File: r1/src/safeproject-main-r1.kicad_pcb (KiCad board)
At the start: 2 copper layers, 29 x 46.5 mm, 18 parts, among them J1 2842142-4, J2 Conn_01x20

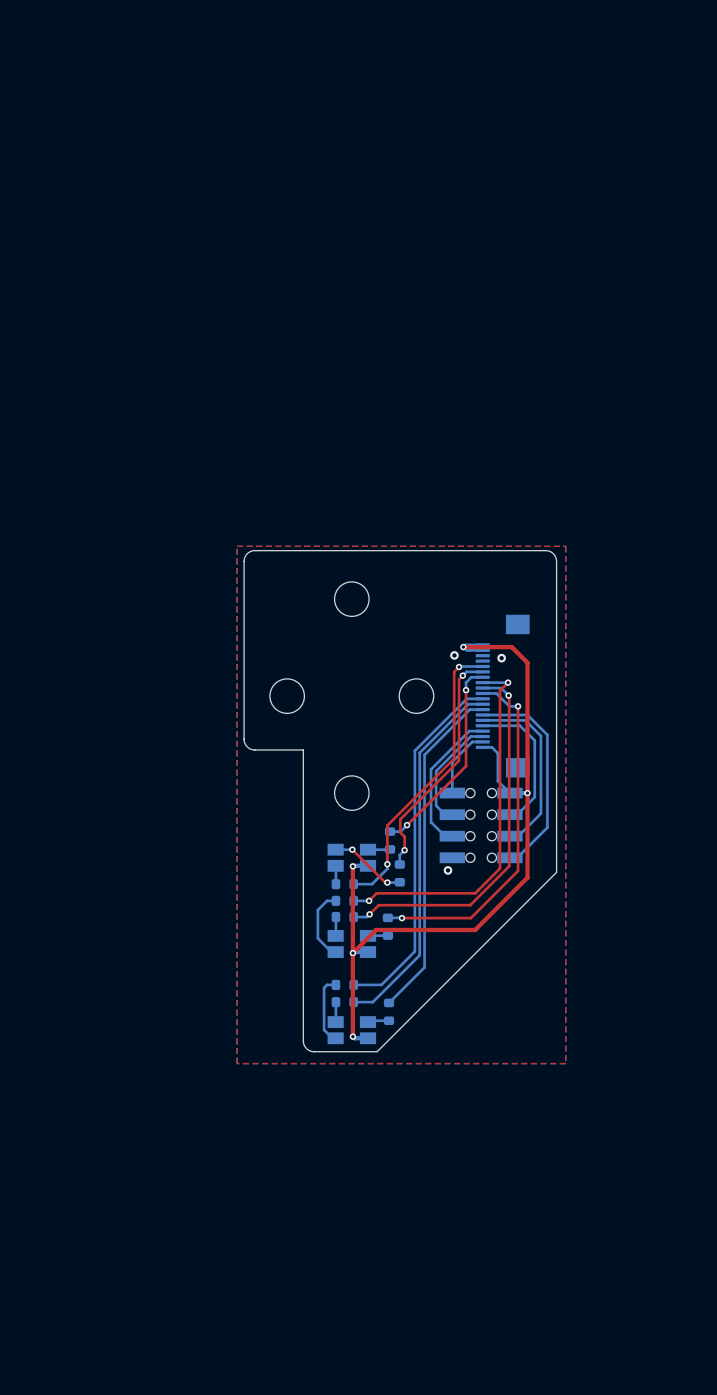
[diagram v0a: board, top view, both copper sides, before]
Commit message: Board routed, DRC pass
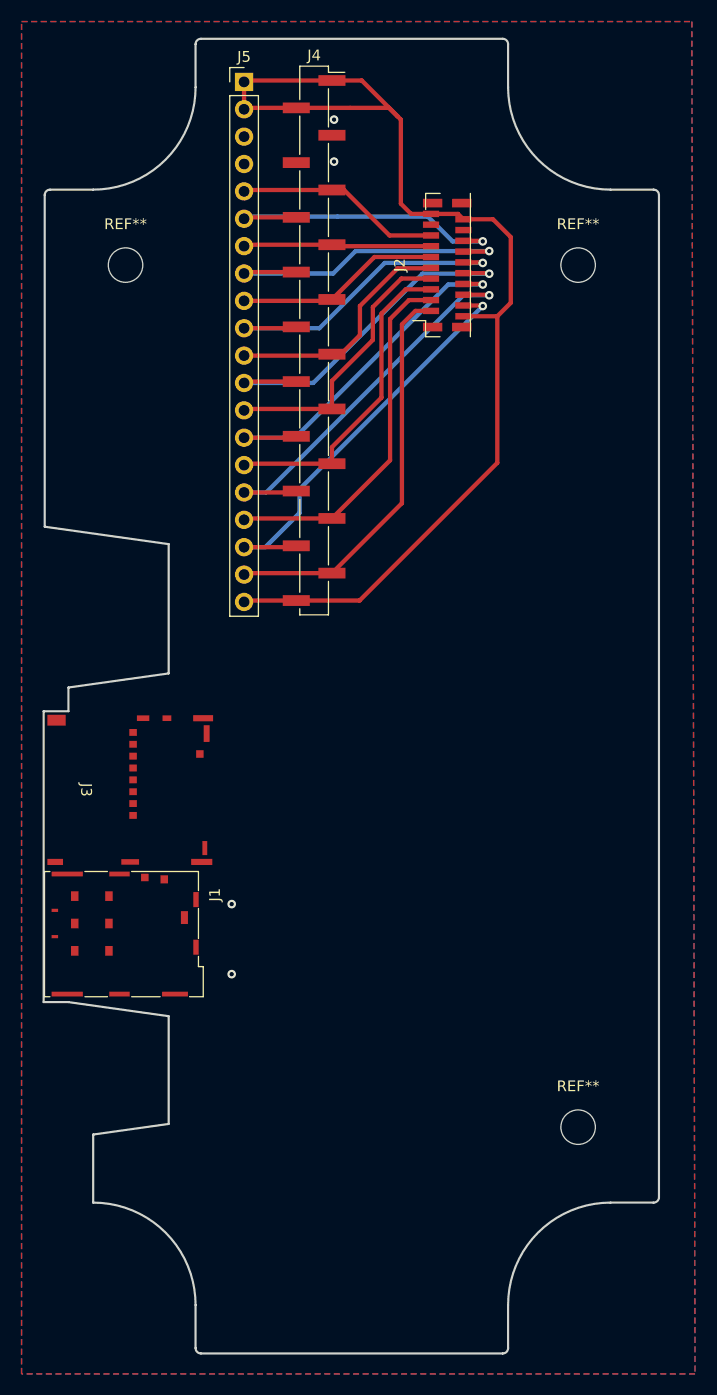
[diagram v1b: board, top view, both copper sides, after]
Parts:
- removed LED1, LED2, LED3: IN-P32TATRGB, LED_SMD:LED_Avago_PLCC4_3.2x2.8mm_CW
- removed R1, R2, R3, R4, R5, R6: 22R, Resistor_SMD:R_0603_1608Metric
- removed R7, R8, R9: 100R, Resistor_SMD:R_0603_1608Metric
- removed the REF** at (0.00, 9.00)
- removed the REF** at (6.00, 0.00)
- removed the REF** at (-6.00, 0.00)
- removed the REF** at (0.00, -9.00)
- added J3: Micro_SD_Card_Det_JAE_ST11, jeffmakes-footprints:microSD_JAE_ST11S008V4H, F.Cu at (-28.2, 8.70)
- added J4: Conn_01x20, Connector_PinHeader_2.54mm:PinHeader_1x20_P2.54mm_Vertical_SMD_Pin1Right, F.Cu at (-3.50, -33.0)
- added J5: Conn_01x20, Connector_PinHeader_2.54mm:PinHeader_1x20_P2.54mm_Vertical, F.Cu at (-10.0, -57.0)
- added REF**: MountingHole_3.2mm_M3_DIN965, MountingHole:MountingHole_3.2mm_M3_DIN965, F.Cu at (21.0, 40.0)
- added REF**: MountingHole_3.2mm_M3_DIN965, MountingHole:MountingHole_3.2mm_M3_DIN965, F.Cu at (-21.0, -40.0)
- added REF**: MountingHole_3.2mm_M3_DIN965, MountingHole:MountingHole_3.2mm_M3_DIN965, F.Cu at (21.0, -40.0)
- J1: value 2842142-4 -> JAE_SIM_Card_SF72S006; footprint jeffmakes-footprints:PinSocket_2x04_P2.00mm_Vertical_SMD_Bottom_or_Top_Entry_AMPMODU -> Connector_JAE:JAE_SIM_Card_SF72S006; moved to F.Cu
- J2: footprint Connector_FFC-FPC:Hirose_FH12-20S-0.5SH_1x20-1MP_P0.50mm_Horizontal -> jeffmakes-footprints:Hirose_FH12-20S-0.5SVA_1x20-1MP_P0.50mm_Vertical; moved to F.Cu
- moved J2 40.4 mm to (8.15, -40.0), turned to 90 degrees
- moved J1 36.4 mm to (-23.2, 21.1), turned to 90 degrees
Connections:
- J2 pad 1: +3V3 -> /+3V3
- J2 pad 2: +3V3 -> /+3V3
- J2 pad 20: +3V3 -> /+3V3
- J2 pad 3: GND -> /GND
- J2 pad 4: GND -> /GND
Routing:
- net /+3V3: track 0.00 -> 106.0 mm
- net +3V3: track 77.0 -> 0.00 mm, vias 5 -> 0
- net /SHDNZ: track 6.49 -> 37.2 mm
- net /SCL: track 10.7 -> 39.4 mm, vias 0 -> 1
- net /FSYNC: track 13.6 -> 37.6 mm, vias 0 -> 1
- net /SDA: track 13.7 -> 33.5 mm
- net /LED2_G: track 34.9 -> 19.0 mm, vias 2 -> 0
- net /SDOUT: track 20.0 -> 34.8 mm, vias 0 -> 1
- net /BCLK: track 16.9 -> 29.6 mm
- net /LED3_R: track 33.9 -> 22.3 mm
- net /LED1_R: track 27.4 -> 19.2 mm, vias 2 -> 0
- net /LED1_G: track 22.3 -> 30.0 mm, vias 2 -> 1
- net Net-(LED1-Pad4): track 7.22 -> 0.00 mm, vias 2 -> 0
- net Net-(LED2-Pad1): track 6.84 -> 0.00 mm
- net Net-(LED3-Pad1): track 6.51 -> 0.00 mm
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- added copper zone on B.Cu, net /GND
- added copper zone on F.Cu, net /GND
- removed copper zone on B.Cu, net GND
- removed copper zone on F.Cu, net GND
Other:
- board size 29 x 46.5 mm -> 57.1 x 122 mm
- board text removed: "1"
- board text removed: "3"
- board text removed: "5"
- board text removed: "7"
- board text removed: "safeacoustics-led-r1 Monad 2021"
